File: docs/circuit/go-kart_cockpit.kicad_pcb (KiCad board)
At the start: 2 copper layers, 103.5 x 57.2 mm, 36 parts, among them P1 Power, Q1 IRLIZ44N, X1 Taster rechts (male), X10 Display (male), X11 PD7, X12 SDA PG4, X13 AVR-ISP-10, X14 Taster links (male), X15 Start/Stop/Rückwärts, X2 5V GND, X3 24V Hupe, X4 SCL, X5 CS, X6 PB6, X7 J5, X8 J3, X9 Bluetooth-Modul

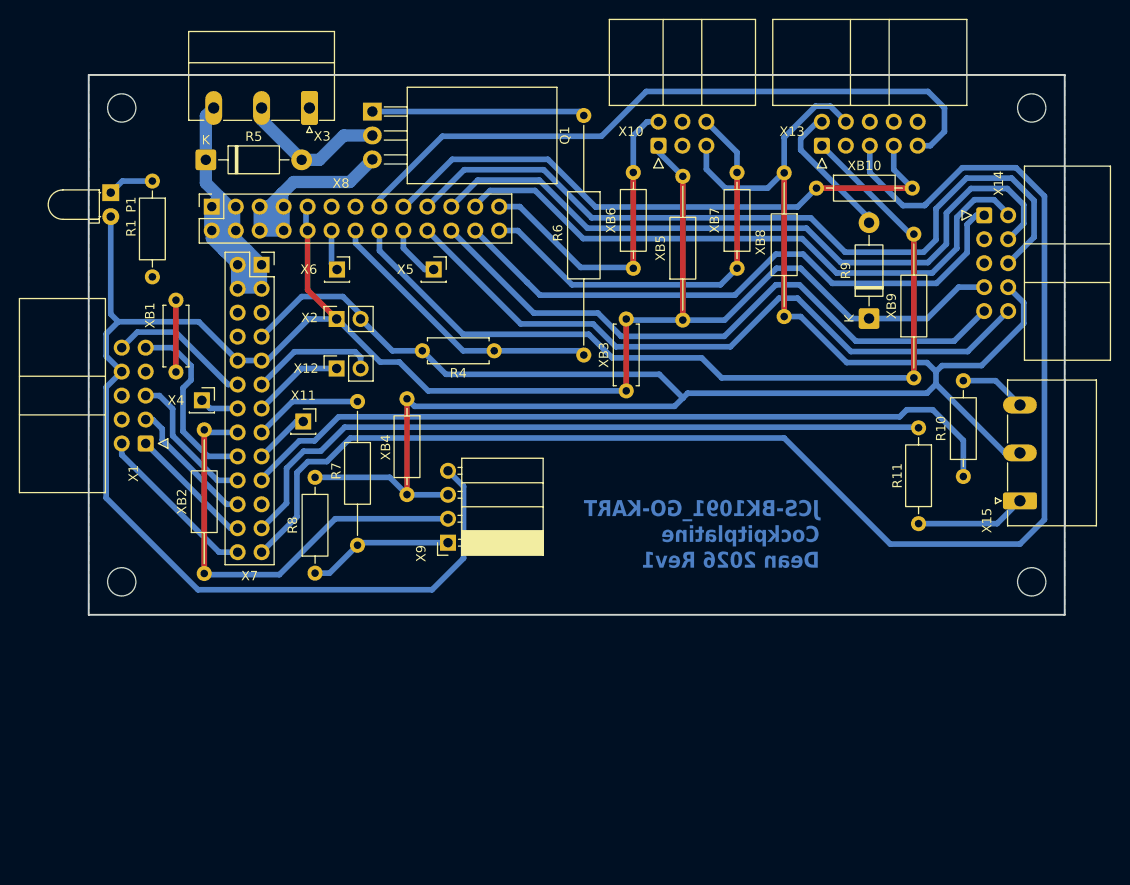
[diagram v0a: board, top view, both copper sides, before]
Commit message: feat: rework of PCB, fix wrong connection
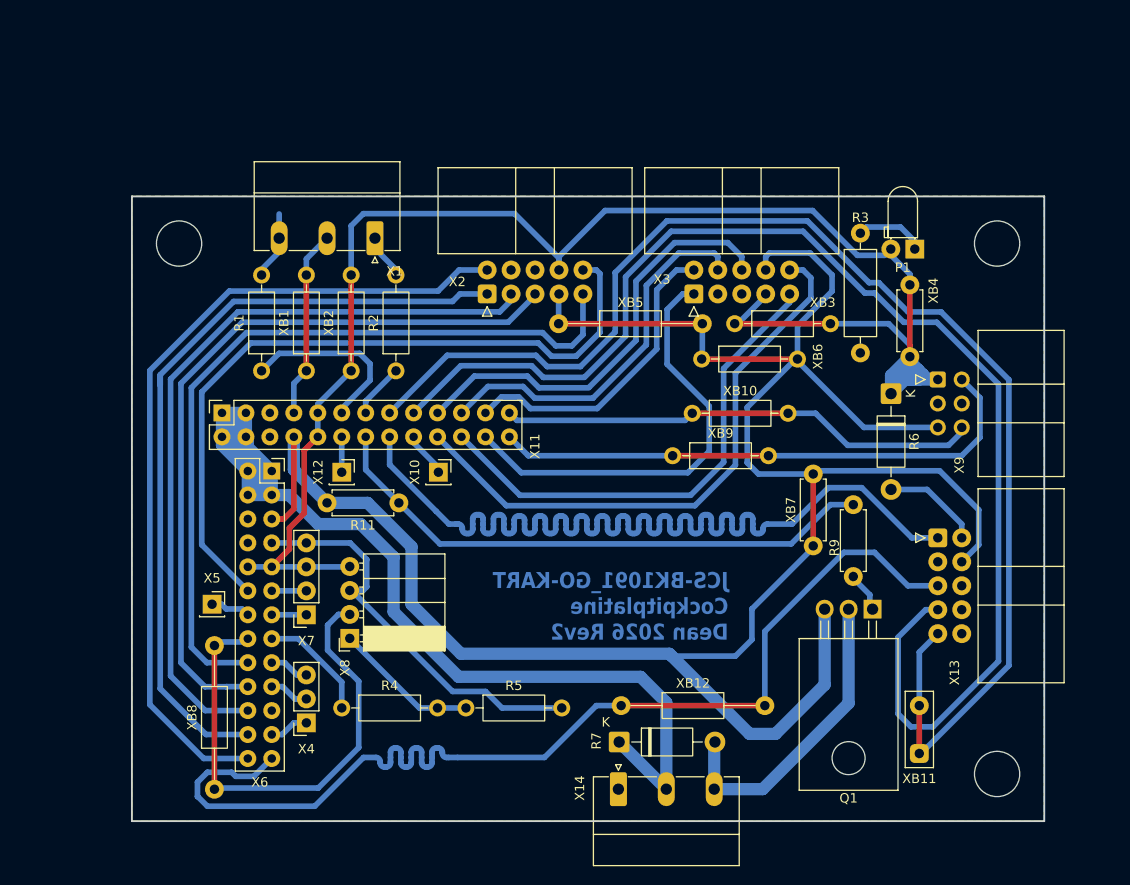
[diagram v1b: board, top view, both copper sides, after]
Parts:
- removed R10: 100, Resistor_THT:R_Axial_DIN0207_L6.3mm_D2.5mm_P10.16mm_Horizontal
- removed the R7 at (67.7, 62.8)
- removed R8: 5.6k, Resistor_THT:R_Axial_DIN0207_L6.3mm_D2.5mm_P10.16mm_Horizontal
- removed the X11 at (61.9, 64.9)
- removed the X2 at (65.5, 54.0)
- removed the X6 at (65.5, 48.8)
- added R2: 100, Resistor_THT:R_Axial_DIN0207_L6.3mm_D2.5mm_P10.16mm_Horizontal, F.Cu at (71.8, 59.5)
- added R3: 820, Resistor_THT:R_Axial_DIN0309_L9.0mm_D3.2mm_P12.70mm_Horizontal, F.Cu at (121.0, 44.9)
- added R5: 5.6k, Resistor_THT:R_Axial_DIN0207_L6.3mm_D2.5mm_P10.16mm_Horizontal, F.Cu at (79.2, 95.2)
- added X10: CS, Connector_PinSocket_2.54mm:PinSocket_1x01_P2.54mm_Vertical, F.Cu at (76.2, 70.2)
- added X7: PD1 PG4 VCC GND, Connector_PinSocket_2.54mm:PinSocket_1x04_P2.54mm_Vertical, F.Cu at (62.2, 85.4)
- added XB11: MISO, TestPoint:TestPoint_2Pads_Pitch5.08mm_Drill1.3mm, F.Cu at (127.2, 100.1)
- added XB12: /RESET, Resistor_THT:R_Axial_DIN0207_L6.3mm_D2.5mm_P15.24mm_Horizontal, F.Cu at (95.6, 95.0)
- Q1: value IRLIZ44N -> IRL3803; footprint Library:TO-220-3_Horizontal_TabDown_no_hole -> Package_TO_SOT_THT:TO-220F-3_Horizontal_TabDown
- R1: value 820 -> 100
- R11: value 100 -> 10k; footprint Resistor_THT:R_Axial_DIN0207_L6.3mm_D2.5mm_P10.16mm_Horizontal -> Resistor_THT:R_Axial_DIN0207_L6.3mm_D2.5mm_P7.62mm_Horizontal
- R4: value 10k -> 3.3k; footprint Resistor_THT:R_Axial_DIN0207_L6.3mm_D2.5mm_P7.62mm_Horizontal -> Resistor_THT:R_Axial_DIN0207_L6.3mm_D2.5mm_P10.16mm_Horizontal
- R6: value 100 -> 1N5817; footprint Resistor_THT:R_Axial_DIN0309_L9.0mm_D3.2mm_P25.40mm_Horizontal -> Diode_THT:D_DO-41_SOD81_P10.16mm_Horizontal
- R9: value 1N5817 -> 100; footprint Diode_THT:D_DO-41_SOD81_P10.16mm_Horizontal -> Resistor_THT:R_Axial_DIN0207_L6.3mm_D2.5mm_P7.62mm_Horizontal
- X12: value SDA PG4 -> PB6; footprint Connector_PinSocket_2.54mm:PinSocket_1x02_P2.54mm_Vertical -> Connector_PinSocket_2.54mm:PinSocket_1x01_P2.54mm_Vertical
- X4: value SCL -> PC2 PG1 PD7; footprint Connector_PinSocket_2.54mm:PinSocket_1x01_P2.54mm_Vertical -> Connector_PinSocket_2.54mm:PinSocket_1x03_P2.54mm_Vertical
- X5: value CS -> SCL
- XB1: footprint Resistor_THT:R_Axial_DIN0207_L6.3mm_D2.5mm_P7.62mm_Horizontal -> Resistor_THT:R_Axial_DIN0207_L6.3mm_D2.5mm_P10.16mm_Horizontal
- XB10: value ISP_SCK -> TXD0
- XB2: value ~ -> Vcc; footprint Resistor_THT:R_Axial_DIN0207_L6.3mm_D2.5mm_P15.24mm_Horizontal -> Resistor_THT:R_Axial_DIN0207_L6.3mm_D2.5mm_P10.16mm_Horizontal
- XB3: value Display_Vcc -> Vcc; footprint Resistor_THT:R_Axial_DIN0207_L6.3mm_D2.5mm_P7.62mm_Horizontal -> Resistor_THT:R_Axial_DIN0207_L6.3mm_D2.5mm_P10.16mm_Horizontal
- XB4: value Display_GND -> Vcc; footprint Resistor_THT:R_Axial_DIN0207_L6.3mm_D2.5mm_P10.16mm_Horizontal -> Resistor_THT:R_Axial_DIN0207_L6.3mm_D2.5mm_P7.62mm_Horizontal
- XB5: value Display_Vcc -> GND
- XB6: value TXD0 -> GND
- XB7: value RXD0 -> GND; footprint Resistor_THT:R_Axial_DIN0207_L6.3mm_D2.5mm_P10.16mm_Horizontal -> Resistor_THT:R_Axial_DIN0207_L6.3mm_D2.5mm_P7.62mm_Horizontal
- XB8: value GND -> ~
- XB9: value ISP_MOSI -> RXD0; footprint Resistor_THT:R_Axial_DIN0207_L6.3mm_D2.5mm_P15.24mm_Horizontal -> Resistor_THT:R_Axial_DIN0207_L6.3mm_D2.5mm_P10.16mm_Horizontal
- moved XB8 89.0 mm to (52.5, 103.9), turned to 90 degrees
- moved P1 85.5 mm to (126.8, 46.6), turned to 180 degrees
- moved X14 79.3 mm to (95.3, 103.9), turned to 0 degrees
- moved R7 75.7 mm to (95.4, 98.9)
- moved Q1 74.8 mm to (122.3, 84.8), turned to 180 degrees
- moved X1 73.8 mm to (69.5, 45.4), turned to 180 degrees
- moved R11 55.7 mm to (72.1, 73.5), turned to 180 degrees
- moved XB4 53.5 mm to (126.2, 58.0), turned to 90 degrees
- moved R6 43.9 mm to (124.2, 61.9)
- moved X13 43.4 mm to (129.2, 77.2), turned to 0 degrees
- moved X5 42.6 mm to (52.2, 84.2)
- moved R4 41.2 mm to (66.0, 95.2), turned to 0 degrees
- moved X2 39.5 mm to (81.4, 51.3), turned to 90 degrees
- moved X9 38.6 mm to (129.2, 60.4), turned to 0 degrees
- moved X4 36.0 mm to (62.2, 96.8), turned to 180 degrees
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- renumbered R5 to R7, X15 to X1, X8 to X11, X3 to X14, X1 to X2, X14 to X3, X7 to X6, X9 to X8, X10 to X9
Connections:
- R1 pad 1: Net-(P1-K) -> /PB7_SW_Reverse
- R1 pad 2: GND -> Net-(X1-4)
- R11 pad 1: /PC2_SW_Start -> PB4_OC2A
- R11 pad 2: Net-(R11-Pad2) -> GND
- R4 pad 1: PB4_OC2A -> PD3_TXD1
- R4 pad 2: GND -> /BL_RX3V3
- R6 pad 1: Net-(Q1-G) -> Vcc (5V)
- R6 pad 2: PB4_OC2A -> Net-(R6-A)
- R9 pad 1: Vcc (5V) -> Net-(Q1-G)
- R9 pad 2: Net-(R9-A) -> PB4_OC2A
- X1 pad 1: Net-(R11-Pad2) -> Net-(R2-Pad2)
- X1 pad 3: Net-(X15-4) -> Net-(X1-4)
- X11 pad 11: unconnected-(X8-Pin_11-Pad11) -> /PB7_SW_Reverse
- X11 pad 13: unconnected-(X8-Pin_13-Pad13) -> /PB5_SW_Start
- X12 pad 1: /PD1_SDA -> /PB6_OC1B
- X13 pad 2: Net-(R9-A) -> Net-(R6-A)
- X14 pad 2: /Hupe (-) -> +24V
- X14 pad 3: +24V -> /Hupe (-)
- X4 pad 1: /PD0_SCL -> /PC2
- X5 pad 1: /PB0_CS -> /PD0_SCL
- X6 pad 19: /PG1_SW_Reverse -> /PG1
- X6 pad 23: /PC2_SW_Start -> /PC2
- X9 pad 2: PE1_TXD0 -> PE0_RXD0
- X9 pad 6: PE0_RXD0 -> PE1_TXD0
- XB10 pad 1: PB1_SCK -> PE1_TXD0
- XB10 pad 2: PB1_SCK -> PE1_TXD0
- XB2 pad 1: PD2_RXD1 -> Vcc (5V)
- XB2 pad 2: PD2_RXD1 -> Vcc (5V)
- XB4 pad 1: GND -> Vcc (5V)
- XB4 pad 2: GND -> Vcc (5V)
- XB5 pad 1: Vcc (5V) -> GND
- XB5 pad 2: Vcc (5V) -> GND
- XB6 pad 1: PE1_TXD0 -> GND
- XB6 pad 2: PE1_TXD0 -> GND
- XB7 pad 1: PE0_RXD0 -> GND
- XB7 pad 2: PE0_RXD0 -> GND
- XB8 pad 1: GND -> PD2_RXD1
- XB8 pad 2: GND -> PD2_RXD1
- XB9 pad 1: PB2_MOSI -> PE0_RXD0
- XB9 pad 2: PB2_MOSI -> PE0_RXD0
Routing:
- net /PG1_SW_Reverse: track 84.1 -> 0.00 mm
- net /PC2_SW_Start: track 76.3 -> 0.00 mm
- net PB1_SCK: track 64.3 -> 138.4 mm
- net PC0_SW_BlinkerR: track 13.5 -> 84.5 mm
- net PB3_MISO: track 72.1 -> 143.0 mm
- net PC3_LED_BlinkerR: track 17.8 -> 88.4 mm
- net PG2_SW_GearDown: track 14.2 -> 81.4 mm
- net PG0_SW_GearUp: track 15.1 -> 79.3 mm
- net PD4_LED_GearUp: track 19.8 -> 83.5 mm
- net PG3_LED_GearDown: track 15.3 -> 77.3 mm
- net +24V: track 69.4 -> 129.9 mm
- net Vcc (5V): track 231.5 -> 179.9 mm
- net GND: track 261.8 -> 305.9 mm
- net /RESET: track 156.6 -> 116.1 mm
- net PE7_SW_Warnblinker: track 83.5 -> 46.4 mm
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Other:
- board size 103.5 x 57.2 mm -> 96.8 x 66.2 mm
- board text added: "DSUB9-CAN"
- board text added: "JCS-BK1091_GO-KART Cockpitplatine Dean 2026 Rev2"
- board text added: "M2"
- board text removed: "JCS-BK1091_GO-KART Cockpitplatine Dean 2026 Rev1"
